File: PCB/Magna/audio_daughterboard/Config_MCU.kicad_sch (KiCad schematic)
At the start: 1 part, among them U1306 STM32F030C8Tx

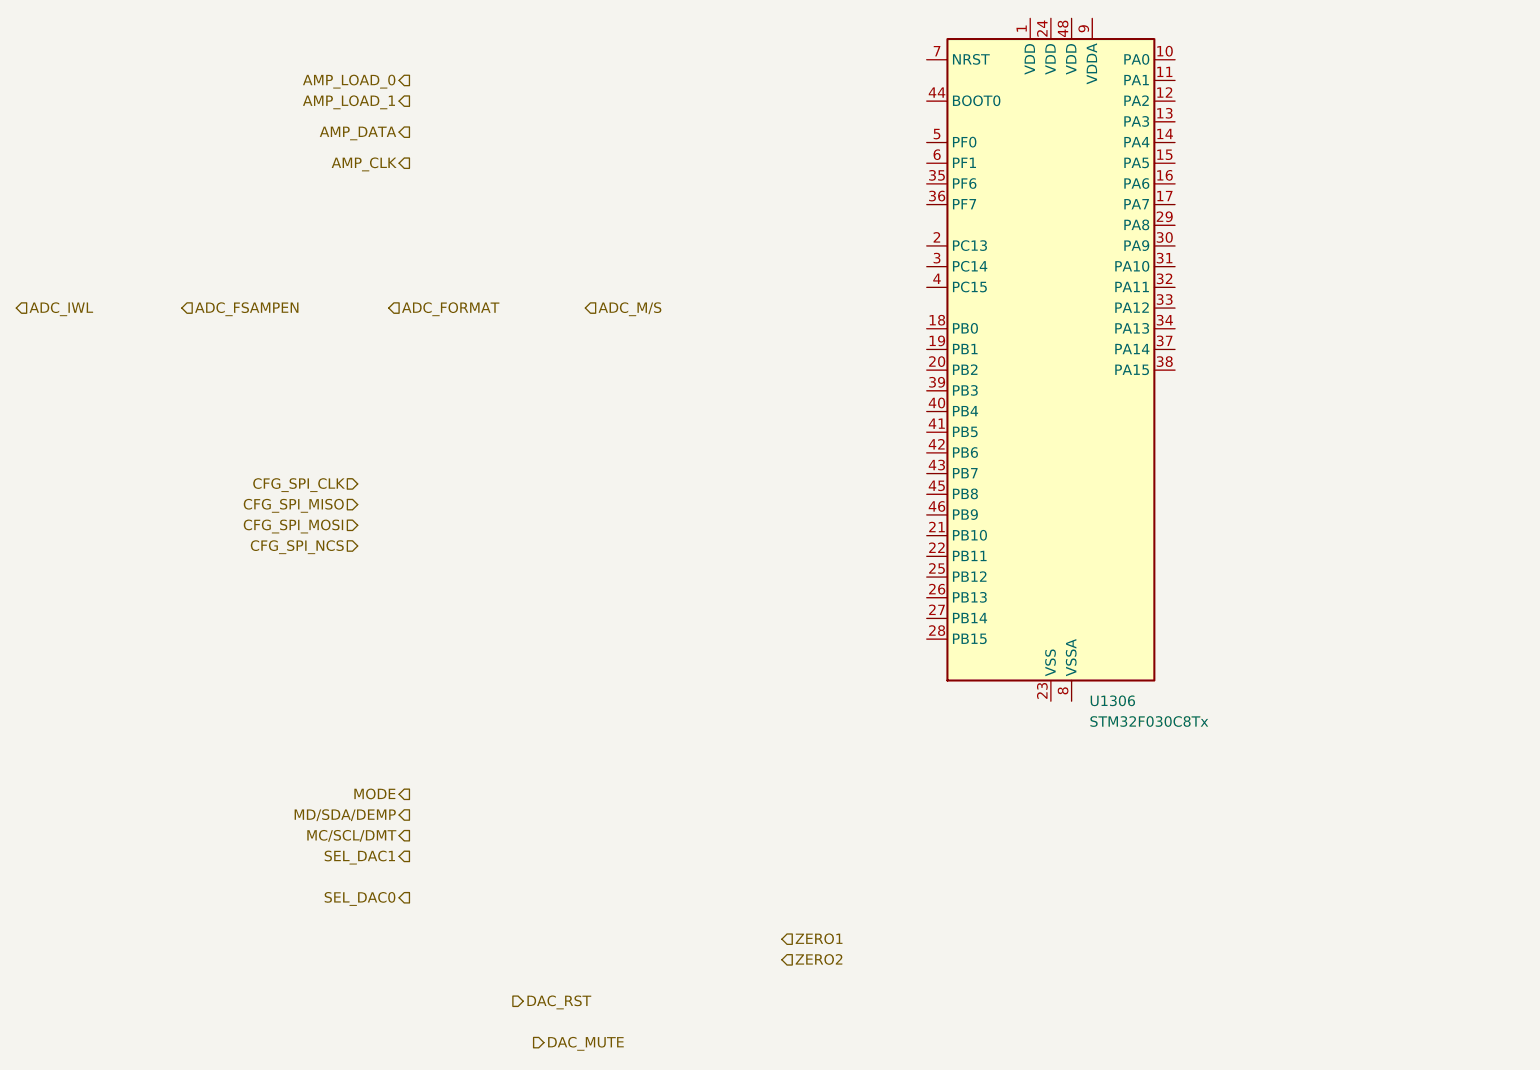
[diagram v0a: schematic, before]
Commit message: Some updates to PCB
Honestly I cannot remember whats changed
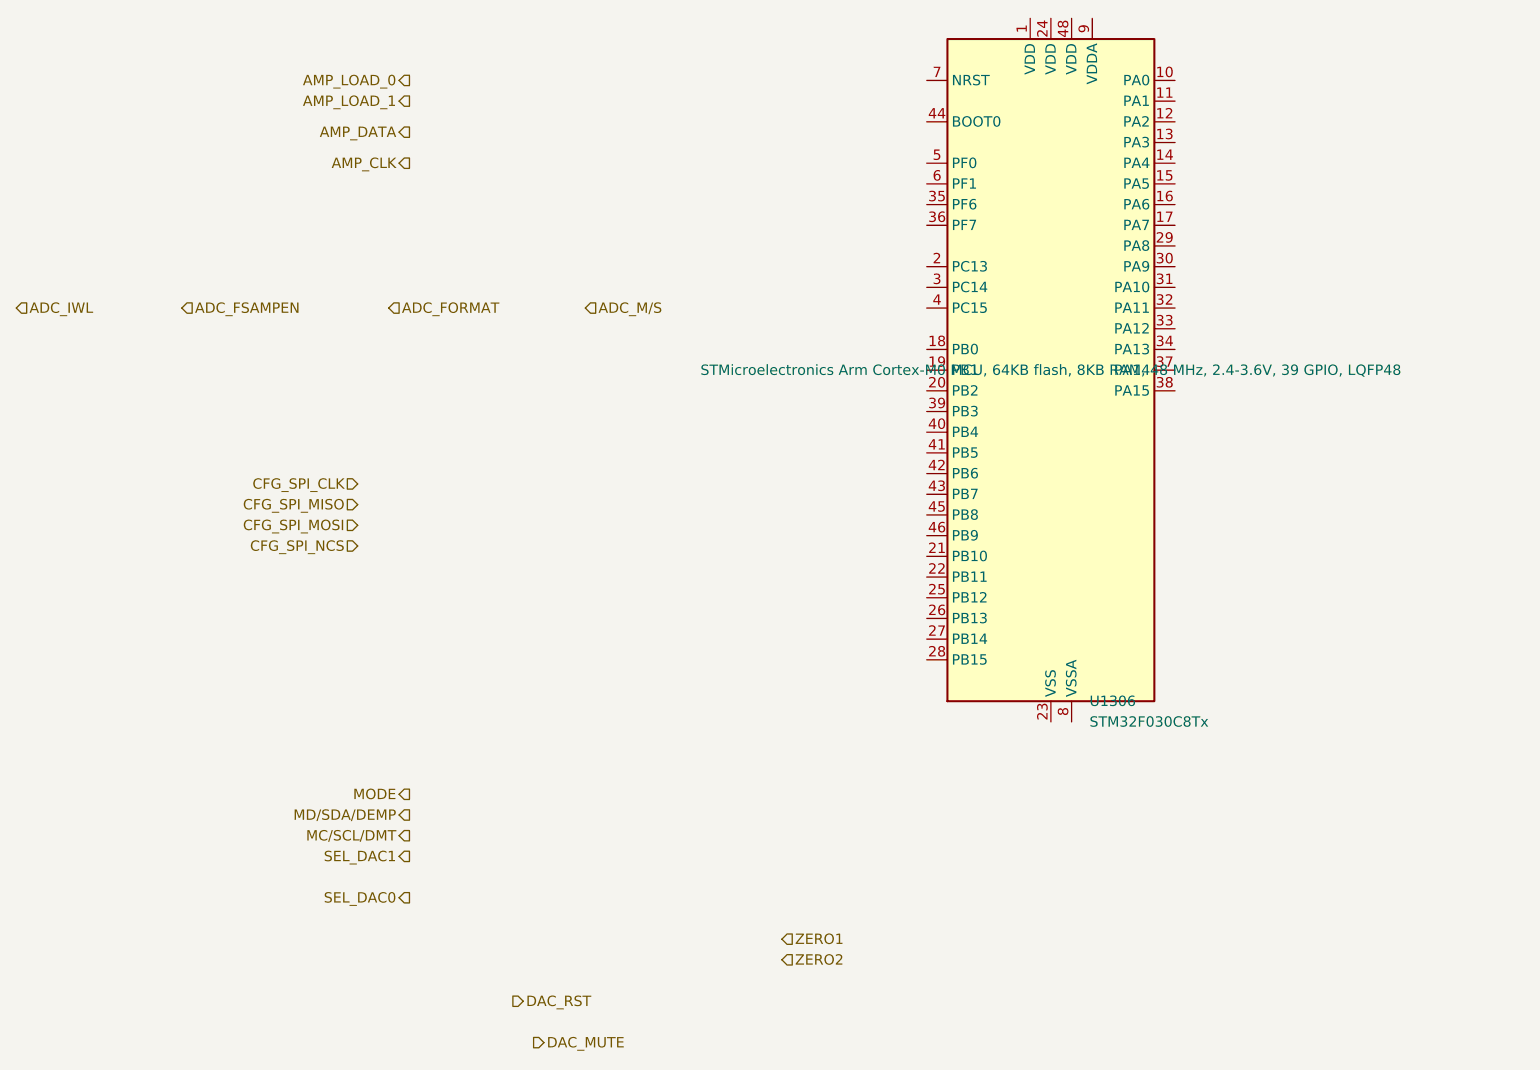
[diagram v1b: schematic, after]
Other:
- moved on the sheet: U1306
